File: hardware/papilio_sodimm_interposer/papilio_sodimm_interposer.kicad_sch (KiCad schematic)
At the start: 1 part, among them U1 Papilio Pro

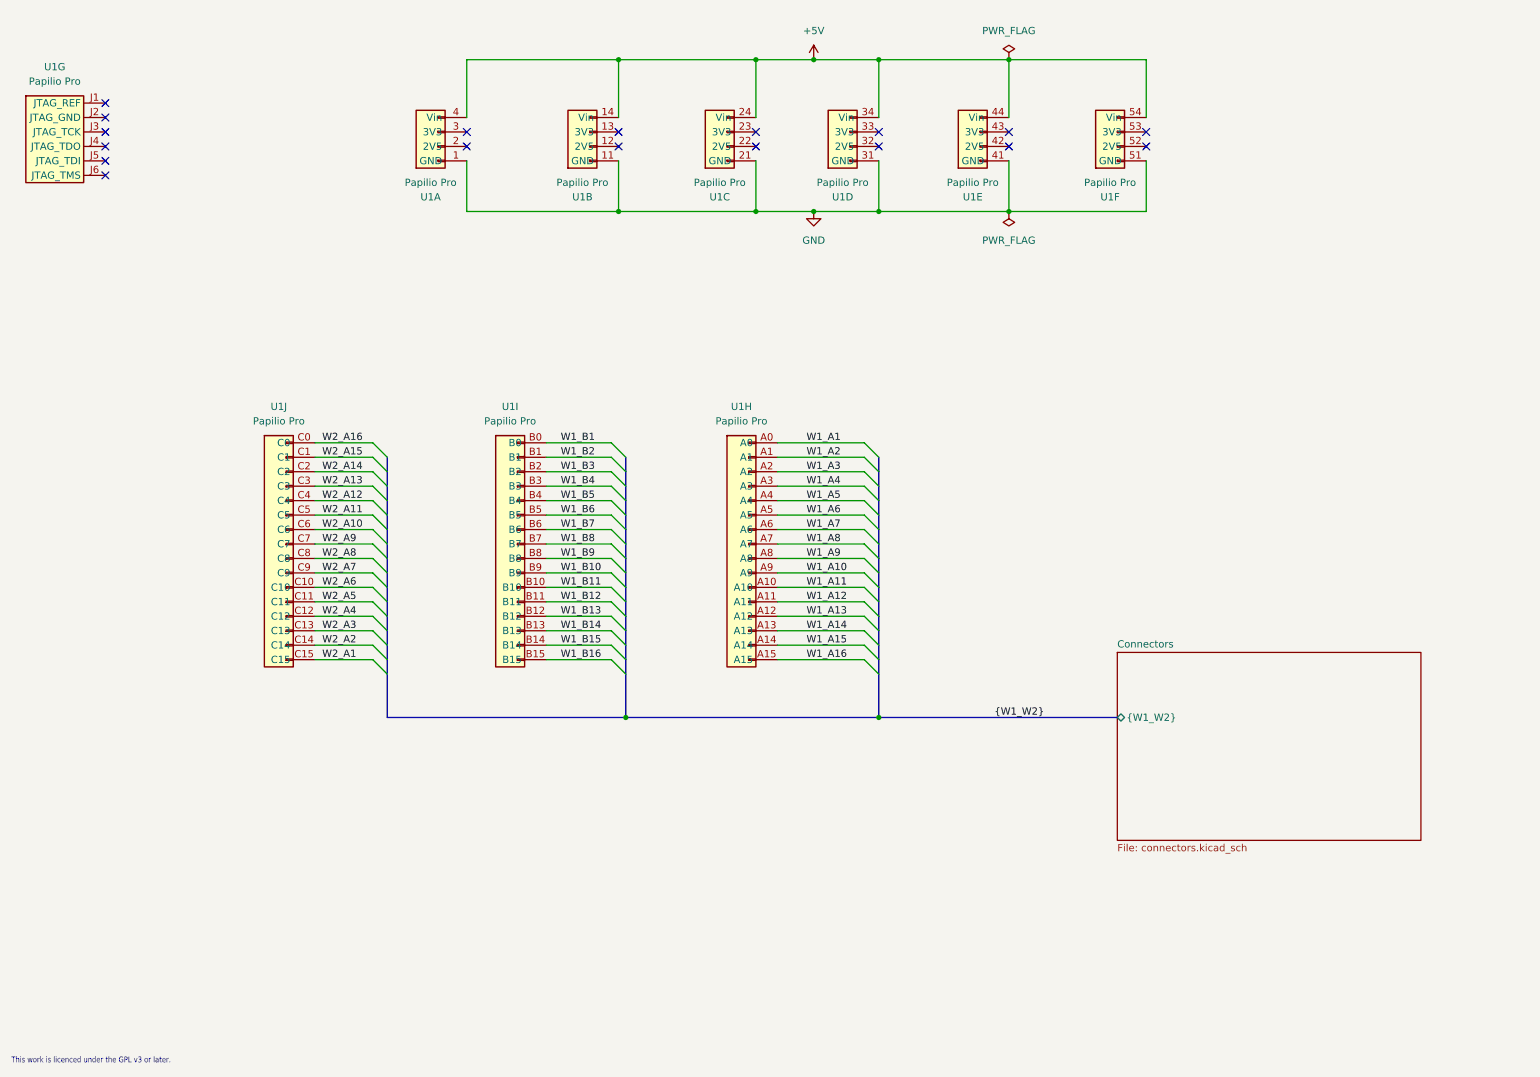
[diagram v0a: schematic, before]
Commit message: Got it going
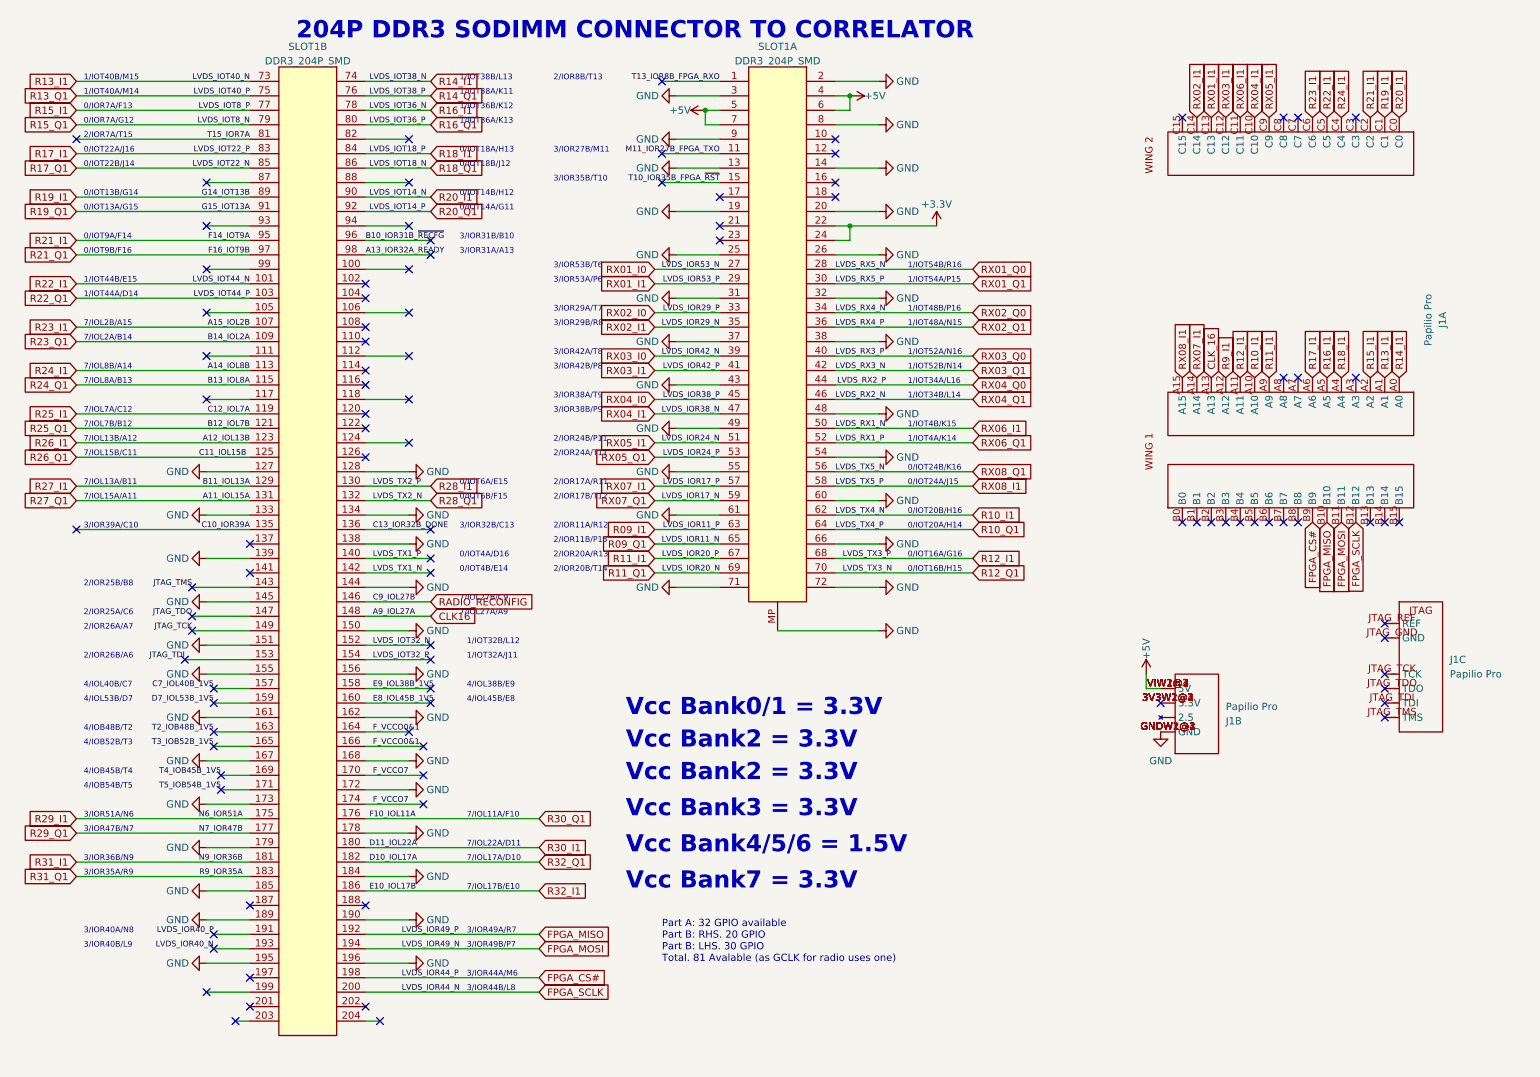
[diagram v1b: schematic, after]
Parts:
- removed U1: Papilio Pro, papilo_pro:COCOON_48BIT, symbol Papilio_Pro:Papilio_Pro
- added J1: Papilio Pro, Papilio_Pro:PAPILIO_PRO, symbol Papilio_pro:Papilio_Pro
- added SLOT1: DDR3_204P_SMD, Papilio_Pro:SODIMM_DDR3_EDGE, symbol Things:DDR3_204P_SMD
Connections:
- net +5V: now also J1.VIW1@1 (5V), J1.VIW1@2 (5V), J1.VIW1@3 (5V), J1.VIW1@4 (5V), J1.VIW2@1 (5V), J1.VIW2@2 (5V), SLOT1.4, SLOT1.5, SLOT1.6, SLOT1.7
- net GND: now also J1.GNDW1@1 (GND), J1.GNDW1@2 (GND), J1.GNDW1@3 (GND), J1.GNDW1@4 (GND), J1.GNDW2@1 (GND), J1.GNDW2@2 (GND), SLOT1.127, SLOT1.128, SLOT1.13, SLOT1.133, SLOT1.134, SLOT1.138, SLOT1.139, SLOT1.14, SLOT1.144, SLOT1.145, SLOT1.150, SLOT1.151, SLOT1.155, SLOT1.156, SLOT1.161, SLOT1.162, SLOT1.167, SLOT1.168, SLOT1.172, SLOT1.173, SLOT1.178, SLOT1.179, SLOT1.184, SLOT1.185, SLOT1.189, SLOT1.19, SLOT1.190, SLOT1.195, SLOT1.196, SLOT1.2, SLOT1.20, SLOT1.25, SLOT1.26, SLOT1.3, SLOT1.31, SLOT1.32, SLOT1.37, SLOT1.38, SLOT1.43, SLOT1.48, SLOT1.49, SLOT1.54, SLOT1.55, SLOT1.60, SLOT1.61, SLOT1.66, SLOT1.71, SLOT1.72, SLOT1.8, SLOT1.9, SLOT1.MP
- new net: J1.3V3W1@1 (3.3V), J1.3V3W1@2 (3.3V), J1.3V3W1@3 (3.3V), J1.3V3W1@4 (3.3V), J1.3V3W2@1 (3.3V), J1.3V3W2@2 (3.3V)
- new net +3.3V: SLOT1.22, SLOT1.24
- new net A13_IOR32A_READY: SLOT1.98
- new net B10_IOR31B_~{RECFG}: SLOT1.96
- new net C10_IOR39A: SLOT1.135
- new net C13_IOR32B_DONE: SLOT1.136
- new net C7_IOL40B_1V5: SLOT1.157
- new net CLK16: SLOT1.148
- new net CLK_16: J1.A13
- new net D7_IOL53B_1V5: SLOT1.159
- new net E8_IOL45B_1V5: SLOT1.160
- new net E9_IOL38B_1V5: SLOT1.158
- new net FPGA_CS#: J1.B9, SLOT1.198
- new net FPGA_MISO: J1.B10, SLOT1.192
- new net FPGA_MOSI: J1.B11, SLOT1.194
- new net FPGA_SCLK: J1.B12, SLOT1.200
- new net F_VCCO0&1: SLOT1.164, SLOT1.166
- new net F_VCCO7: SLOT1.170, SLOT1.174
- new net JTAG_TCK: SLOT1.149
- new net JTAG_TDI: SLOT1.153
- new net JTAG_TDO: SLOT1.147
- new net JTAG_TMS: SLOT1.143
- new net LVDS_IOR40_N: SLOT1.193
- new net LVDS_IOR40_P: SLOT1.191
- new net LVDS_IOT32_N: SLOT1.152
- new net LVDS_IOT32_P: SLOT1.154
- new net LVDS_TX1_N: SLOT1.142
- new net LVDS_TX1_P: SLOT1.140
- new net M11_IOR27B_FPGA_TXO: SLOT1.11
- new net R09_I1: SLOT1.63
- new net R09_Q1: SLOT1.65
- new net R10_I1: J1.A10, SLOT1.62
- new net R10_Q1: SLOT1.64
- new net R11_I1: J1.A9, SLOT1.67
- new net R11_Q1: SLOT1.69
- new net R12_I1: J1.A11, SLOT1.68
- new net R12_Q1: SLOT1.70
- new net R13_I1: J1.A1, SLOT1.73
- new net R13_Q1: SLOT1.75
- new net R14_I1: J1.A0, SLOT1.74
- new net R14_Q1: SLOT1.76
- new net R15_I1: J1.A2, SLOT1.77
- new net R15_Q1: SLOT1.79
- new net R16_I1: J1.A5, SLOT1.78
- new net R16_Q1: SLOT1.80
- new net R17_I1: J1.A6, SLOT1.83
- new net R17_Q1: SLOT1.85
- new net R18_I1: J1.A4, SLOT1.84
- new net R18_Q1: SLOT1.86
- new net R19_I1: J1.C1, SLOT1.89
- new net R19_Q1: SLOT1.91
- new net R20_I1: J1.C0, SLOT1.90
- new net R20_Q1: SLOT1.92
- new net R21_I1: J1.C2, SLOT1.95
- new net R21_Q1: SLOT1.97
- new net R22_I1: J1.C5, SLOT1.101
- new net R22_Q1: SLOT1.103
- new net R23_I1: J1.C6, SLOT1.107
- new net R23_Q1: SLOT1.109
- new net R24_I1: J1.C4, SLOT1.113
- new net R24_Q1: SLOT1.115
- new net R25_I1: SLOT1.119
- new net R25_Q1: SLOT1.121
- new net R26_I1: SLOT1.123
- new net R26_Q1: SLOT1.125
- new net R27_I1: SLOT1.129
- new net R27_Q1: SLOT1.131
- new net R28_I1: SLOT1.130
- new net R28_Q1: SLOT1.132
- new net R29_I1: SLOT1.175
- new net R29_Q1: SLOT1.177
- new net R30_I1: SLOT1.180
- new net R30_Q1: SLOT1.176
- new net R31_I1: SLOT1.181
- new net R31_Q1: SLOT1.183
- new net R32_I1: SLOT1.186
- new net R32_Q1: SLOT1.182
- new net R9_I1: J1.A12
- new net RADIO_RECONFIG: SLOT1.146
- new net RX01_I0: SLOT1.27
- new net RX01_I1: J1.C13, SLOT1.29
- new net RX01_Q0: SLOT1.28
- new net RX01_Q1: SLOT1.30
- new net RX02_I0: SLOT1.33
- new net RX02_I1: J1.C14, SLOT1.35
- new net RX02_Q0: SLOT1.34
- new net RX02_Q1: SLOT1.36
- new net RX03_I0: SLOT1.39
- new net RX03_I1: J1.C12, SLOT1.41
- new net RX03_Q0: SLOT1.40
- new net RX03_Q1: SLOT1.42
- new net RX04_I0: SLOT1.45
- new net RX04_I1: J1.C10, SLOT1.47
- new net RX04_Q0: SLOT1.44
- new net RX04_Q1: SLOT1.46
- new net RX05_I1: J1.C9, SLOT1.51
- new net RX05_Q1: SLOT1.53
- new net RX06_I1: J1.C11, SLOT1.50
- new net RX06_Q1: SLOT1.52
- new net RX07_I1: J1.A14, SLOT1.57
- new net RX07_Q1: SLOT1.59
- new net RX08_I1: J1.A15, SLOT1.58
- new net RX08_Q1: SLOT1.56
- new net T10_IOR35B_FPGA_~{RST}: SLOT1.15
- new net T13_IOR8B_FPGA_RXO: SLOT1.1
- new net T15_IOR7A: SLOT1.81
- new net T2_IOB48B_1V5: SLOT1.163
- new net T3_IOB52B_1V5: SLOT1.165
- new net T4_IOB45B_1V5: SLOT1.169
- new net T5_IOB54B_1V5: SLOT1.171
- no-connect marks 18 -> 96
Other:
- removed sheet Connectors
- note added: "0/IOR7A/F13"
- note added: "0/IOR7A/G12"
- note added: "0/IOT13A/G15"
- note added: "0/IOT13B/G14"
- note added: "0/IOT14A/G11"
- note added: "0/IOT14B/H12"
- note added: "0/IOT16A/G16"
- note added: "0/IOT16B/H15"
- note added: "0/IOT18A/H13"
- note added: "0/IOT18B/J12"
- note added: "0/IOT20A/H14"
- note added: "0/IOT20B/H16"
- note added: "0/IOT22A/J16"
- note added: "0/IOT22B/J14"
- note added: "0/IOT24A/J15"
- note added: "0/IOT24B/K16"
- note added: "0/IOT4A/D16"
- note added: "0/IOT4B/E14"
- note added: "0/IOT6A/E15"
- note added: "0/IOT6B/F15"
- note added: "0/IOT9A/F14"
- note added: "0/IOT9B/F16"
- note added: "1/IOT32A/J11"
- note added: "1/IOT32B/L12"
- note added: "1/IOT34A/L16"
- note added: "1/IOT34B/L14"
- note added: "1/IOT36A/K13"
- note added: "1/IOT36B/K12"
- note added: "1/IOT38A/K11"
- note added: "1/IOT38B/L13"
- note added: "1/IOT40A/M14"
- note added: "1/IOT40B/M15"
- note added: "1/IOT44A/D14"
- note added: "1/IOT44B/E15"
- note added: "1/IOT48A/N15"
- note added: "1/IOT48B/P16"
- note added: "1/IOT4A/K14"
- note added: "1/IOT4B/K15"
- note added: "1/IOT52A/N16"
- note added: "1/IOT52B/N14"
- note added: "1/IOT54A/P15"
- note added: "1/IOT54B/R16"
- note added: "2/IOR11A/R12"
- note added: "2/IOR11B/P13"
- note added: "2/IOR17A/R11"
- note added: "2/IOR17B/T12"
- note added: "2/IOR20A/R13"
- note added: "2/IOR20B/T14"
- note added: "2/IOR24A/T11"
- note added: "2/IOR24B/P11"
- note added: "2/IOR25A/C6"
- note added: "2/IOR25B/B8"
- note added: "2/IOR26A/A7"
- note added: "2/IOR26B/A6"
- note added: "2/IOR7A/T15"
- note added: "2/IOR8B/T13"
- note added: "204P DDR3 SODIMM CONNECTOR TO CORRELATOR"
- note added: "3/IOR27B/M11"
- note added: "3/IOR29A/T7"
- note added: "3/IOR29B/R8"
- note added: "3/IOR31A/A13"
- note added: "3/IOR31B/B10"
- note added: "3/IOR32B/C13"
- note added: "3/IOR35A/R9"
- note added: "3/IOR35B/T10"
- note added: "3/IOR36B/N9"
- note added: "3/IOR38A/T9"
- note added: "3/IOR38B/P9"
- note added: "3/IOR39A/C10"
- note added: "3/IOR40A/N8"
- note added: "3/IOR40B/L9"
- note added: "3/IOR42A/T8"
- note added: "3/IOR42B/P8"
- note added: "3/IOR44A/M6"
- note added: "3/IOR44B/L8"
- note added: "3/IOR47B/N7"
- note added: "3/IOR49A/R7"
- note added: "3/IOR49B/P7"
- note added: "3/IOR51A/N6"
- note added: "3/IOR53A/P6"
- note added: "3/IOR53B/T6"
- note added: "4/IOB45B/T4"
- note added: "4/IOB48B/T2"
- note added: "4/IOB52B/T3"
- note added: "4/IOB54B/T5"
- note added: "4/IOL38B/E9"
- note added: "4/IOL40B/C7"
- note added: "4/IOL45B/E8"
- note added: "4/IOL53B/D7"
- note added: "7/IOL11A/F10"
- note added: "7/IOL13A/B11"
- note added: "7/IOL13B/A12"
- note added: "7/IOL15A/A11"
- note added: "7/IOL15B/C11"
- note added: "7/IOL17A/D10"
- note added: "7/IOL17B/E10"
- note added: "7/IOL22A/D11"
- note added: "7/IOL27A/A9"
- note added: "7/IOL27B/C9"
- note added: "7/IOL2A/B14"
- note added: "7/IOL2B/A15"
- note added: "7/IOL7A/C12"
- note added: "7/IOL7B/B12"
- note added: "7/IOL8A/B13"
- note added: "7/IOL8B/A14"
- note added: "Part A: 32 GPIO available Part B: RHS. 20 GPIO Part B: LHS. 30 GPIO Total. 81 Avalable (as GCLK for radio uses one)"
- note added: "Vcc Bank0/1 = 3.3V"
- note added: "Vcc Bank2 = 3.3V"
- note added: "Vcc Bank3 = 3.3V"
- note added: "Vcc Bank4/5/6 = 1.5V"
- note added: "Vcc Bank7 = 3.3V"
- note removed: "This work is licenced under the GPL v3 or later."
